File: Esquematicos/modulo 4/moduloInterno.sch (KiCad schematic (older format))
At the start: 15 parts

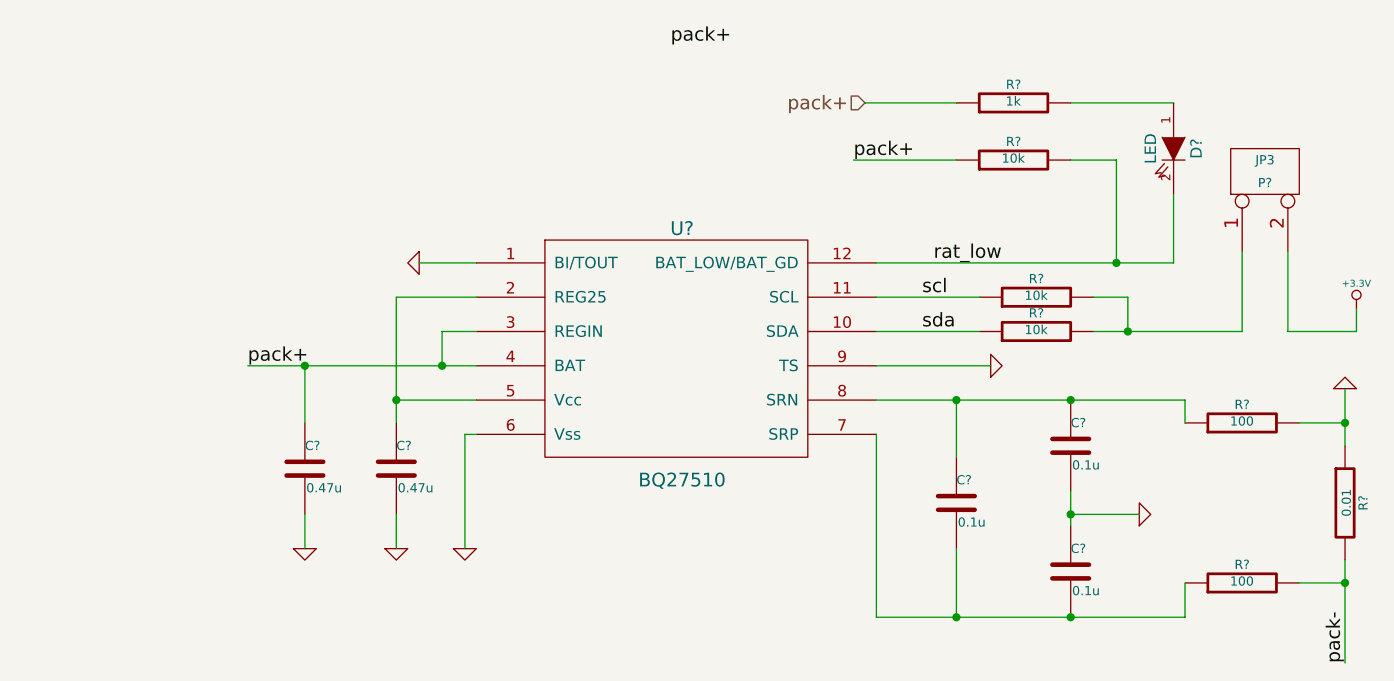
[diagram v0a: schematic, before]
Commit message: Esquematico terminado
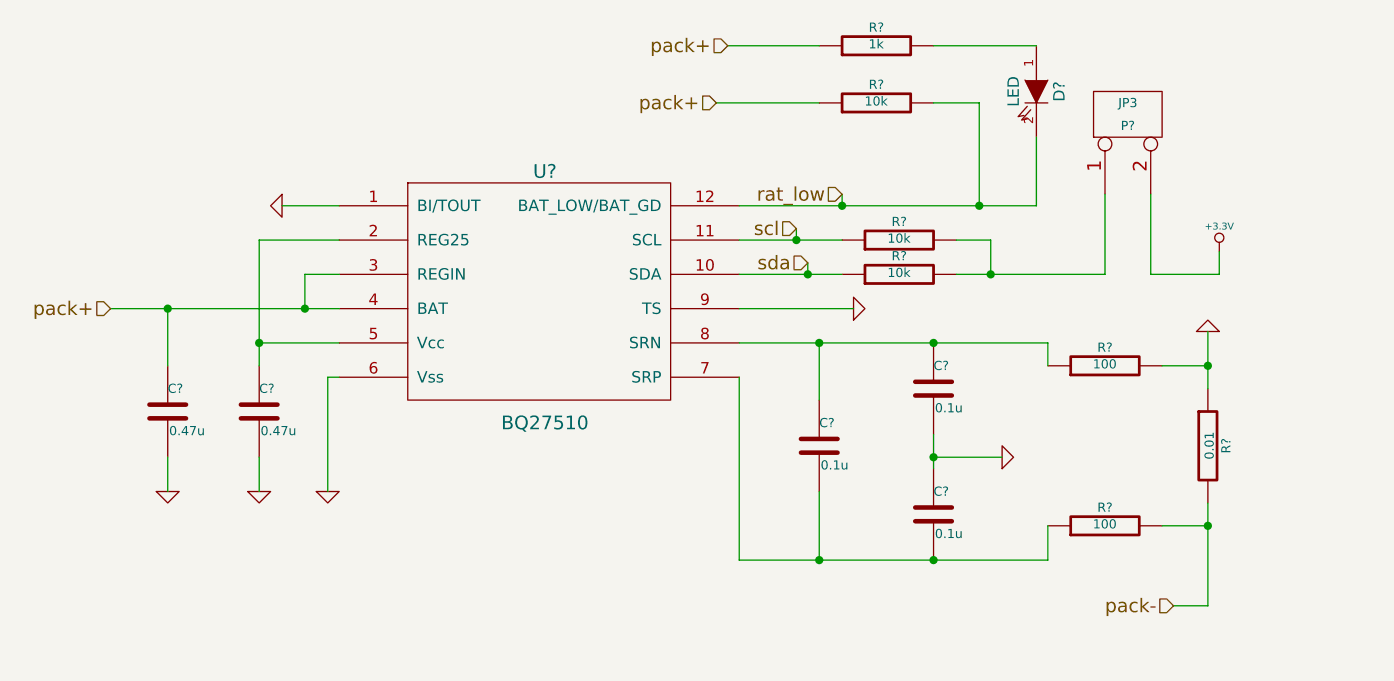
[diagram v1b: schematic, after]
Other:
- moved on the sheet: C?, D?, P?, R?, U?

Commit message: cambios
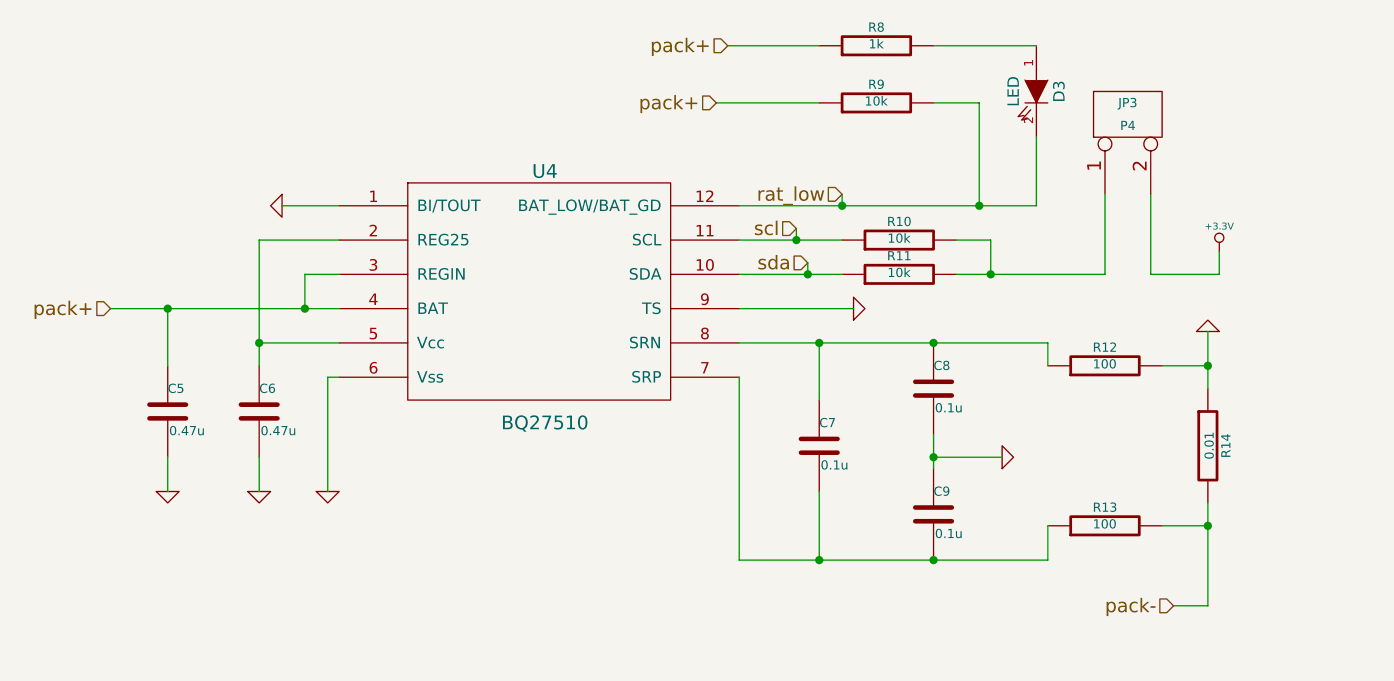
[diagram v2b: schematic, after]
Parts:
- gave numbers to parts that had none: 15
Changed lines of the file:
@@
 Sheet 2 3
 Title ""
-Date "18 feb 2014"
+Date "19 feb 2014"
 Rev ""
 Comp ""
@@
 $EndDescr
 $Comp
-L BQ27510 U?
+L BQ27510 U4
 U 1 1 52FE9FCC
 P 5050 3100
-F 0 "U?" H 5050 3500 60  0000 C CNN
+F 0 "U4" H 5050 3500 60  0000 C CNN
 F 1 "BQ27510" H 5050 2400 60  0000 C CNN
 F 2 "~" H 4850 3150 60  0000 C CNN
@@
 $EndComp
 $Comp
-L GND #PWR?
+L GND #PWR013
 U 1 1 52FE9FCD
 P 3900 2850
-F 0 "#PWR?" H 3900 2850 30  0001 C CNN
+F 0 "#PWR013" H 3900 2850 30  0001 C CNN
 F 1 "GND" H 3900 2780 30  0001 C CNN
 F 2 "" H 3900 2850 60  0000 C CNN
@@
 Connection ~ 4000 3300
 $Comp
-L C C?
+L C C5
 U 1 1 52FE9FCE
 P 3400 3750
-F 0 "C?" H 3400 3850 40  0000 L CNN
+F 0 "C5" H 3400 3850 40  0000 L CNN
 F 1 "0.47u" H 3406 3665 40  0000 L CNN
 F 2 "~" H 3438 3600 30  0000 C CNN
@@
 Connection ~ 3400 3300
 $Comp
-L C C?
+L C C6
 U 1 1 52FE9FCF
 P 3800 3750
-F 0 "C?" H 3800 3850 40  0000 L CNN
+F 0 "C6" H 3800 3850 40  0000 L CNN
 F 1 "0.47u" H 3806 3665 40  0000 L CNN
 F 2 "~" H 3838 3600 30  0000 C CNN
@@
 Connection ~ 3800 3450
 $Comp
-L GND #PWR?
+L GND #PWR014
 U 1 1 52FE9FD0
 P 3400 4100
-F 0 "#PWR?" H 3400 4100 30  0001 C CNN
+F 0 "#PWR014" H 3400 4100 30  0001 C CNN
 F 1 "GND" H 3400 4030 30  0001 C CNN
 F 2 "" H 3400 4100 60  0000 C CNN
@@
 $EndComp
 $Comp
-L GND #PWR?
+L GND #PWR015
 U 1 1 52FE9FD1
 P 3800 4100
-F 0 "#PWR?" H 3800 4100 30  0001 C CNN
+F 0 "#PWR015" H 3800 4100 30  0001 C CNN
 F 1 "GND" H 3800 4030 30  0001 C CNN
 F 2 "" H 3800 4100 60  0000 C CNN
@@
 $EndComp
 $Comp
-L GND #PWR?
+L GND #PWR016
 U 1 1 52FE9FD2
 P 4100 4100
-F 0 "#PWR?" H 4100 4100 30  0001 C CNN
+F 0 "#PWR016" H 4100 4100 30  0001 C CNN
 F 1 "GND" H 4100 4030 30  0001 C CNN
 F 2 "" H 4100 4100 60  0000 C CNN
@@
 	3400 3950 3400 4100
 $Comp
-L R R?
+L R R9
 U 1 1 52FE9FD3
 P 6500 2400
-F 0 "R?" V 6580 2400 40  0000 C CNN
+F 0 "R9" V 6580 2400 40  0000 C CNN
 F 1 "10k" V 6507 2401 40  0000 C CNN
 F 2 "~" V 6430 2400 30  0000 C CNN
@@
 $EndComp
 $Comp
-L R R?
+L R R8
 U 1 1 52FE9FD4
 P 6500 2150
-F 0 "R?" V 6580 2150 40  0000 C CNN
+F 0 "R8" V 6580 2150 40  0000 C CNN
 F 1 "1k" V 6507 2151 40  0000 C CNN
 F 2 "~" V 6430 2150 30  0000 C CNN
@@
 	5800 2400 6250 2400
 $Comp
-L LED D?
+L LED D3
 U 1 1 52FE9FD5
 P 7200 2350
-F 0 "D?" H 7200 2450 50  0000 C CNN
+F 0 "D3" H 7200 2450 50  0000 C CNN
 F 1 "LED" H 7200 2250 50  0000 C CNN
 F 2 "~" H 7200 2350 60  0000 C CNN
@@
 Connection ~ 6950 2850
 $Comp
-L R R?
+L R R10
 U 1 1 52FE9FD6
 P 6600 3000
-F 0 "R?" V 6680 3000 40  0000 C CNN
+F 0 "R10" V 6680 3000 40  0000 C CNN
 F 1 "10k" V 6607 3001 40  0000 C CNN
 F 2 "~" V 6530 3000 30  0000 C CNN
@@
 	5900 3000 6350 3000
 $Comp
-L R R?
+L R R11
 U 1 1 52FE9FD7
 P 6600 3150
-F 0 "R?" V 6680 3150 40  0000 C CNN
+F 0 "R11" V 6680 3150 40  0000 C CNN
 F 1 "10k" V 6607 3151 40  0000 C CNN
 F 2 "~" V 6530 3150 30  0000 C CNN
@@
 	7000 3000 7000 3150
 $Comp
-L CONN_2 P?
+L CONN_2 P4
 U 1 1 52FE9FD8
 P 7600 2450
-F 0 "P?" V 7550 2450 40  0000 C CNN
+F 0 "P4" V 7550 2450 40  0000 C CNN
 F 1 "JP3" V 7650 2450 40  0000 C CNN
 F 2 "" H 7600 2450 60  0000 C CNN
@@
 	7700 3150 8000 3150
 $Comp
-L +3.3V #PWR?
+L +3.3V #PWR017
 U 1 1 52FE9FD9
 P 8000 3050
-F 0 "#PWR?" H 8000 3010 30  0001 C CNN
+F 0 "#PWR017" H 8000 3010 30  0001 C CNN
 F 1 "+3.3V" H 8000 3160 30  0000 C CNN
 F 2 "" H 8000 3050 60  0000 C CNN
@@
 	8000 3150 8000 3050
 $Comp
-L GND #PWR?
+L GND #PWR018
 U 1 1 52FE9FDA
 P 6400 3300
-F 0 "#PWR?" H 6400 3300 30  0001 C CNN
+F 0 "#PWR018" H 6400 3300 30  0001 C CNN
 F 1 "GND" H 6400 3230 30  0001 C CNN
 F 2 "" H 6400 3300 60  0000 C CNN
@@
 	5900 3300 6400 3300
 $Comp
-L C C?
+L C C7
 U 1 1 52FE9FDB
 P 6250 3900
-F 0 "C?" H 6250 4000 40  0000 L CNN
+F 0 "C7" H 6250 4000 40  0000 L CNN
 F 1 "0.1u" H 6256 3815 40  0000 L CNN
 F 2 "~" H 6288 3750 30  0000 C CNN
@@
 	5900 3600 5900 4400
 $Comp
-L C C?
+L C C8
 U 1 1 52FE9FDC
 P 6750 3650
-F 0 "C?" H 6750 3750 40  0000 L CNN
+F 0 "C8" H 6750 3750 40  0000 L CNN
 F 1 "0.1u" H 6756 3565 40  0000 L CNN
 F 2 "~" H 6788 3500 30  0000 C CNN
@@
 Connection ~ 6250 3450
 $Comp
-L C C?
+L C C9
 U 1 1 52FE9FDD
 P 6750 4200
-F 0 "C?" H 6750 4300 40  0000 L CNN
+F 0 "C9" H 6750 4300 40  0000 L CNN
 F 1 "0.1u" H 6756 4115 40  0000 L CNN
 F 2 "~" H 6788 4050 30  0000 C CNN
@@
 	6750 3850 6750 4000
 $Comp
-L GND #PWR?
+L GND #PWR019
 U 1 1 52FE9FDE
 P 7050 3950
-F 0 "#PWR?" H 7050 3950 30  0001 C CNN
+F 0 "#PWR019" H 7050 3950 30  0001 C CNN
 F 1 "GND" H 7050 3880 30  0001 C CNN
 F 2 "" H 7050 3950 60  0000 C CNN
@@
 Connection ~ 6750 3950
 $Comp
-L R R?
+L R R12
 U 1 1 52FE9FDF
 P 7500 3550
-F 0 "R?" V 7580 3550 40  0000 C CNN
+F 0 "R12" V 7580 3550 40  0000 C CNN
 F 1 "100" V 7507 3551 40  0000 C CNN
 F 2 "~" V 7430 3550 30  0000 C CNN
@@
 $EndComp
 $Comp
-L R R?
+L R R13
 U 1 1 52FE9FE0
 P 7500 4250
-F 0 "R?" V 7580 4250 40  0000 C CNN
+F 0 "R13" V 7580 4250 40  0000 C CNN
 F 1 "100" V 7507 4251 40  0000 C CNN
 F 2 "~" V 7430 4250 30  0000 C CNN
@@
 Connection ~ 6750 3450
 $Comp
-L R R?
+L R R14
 U 1 1 52FE9FE1
 P 7950 3900
-F 0 "R?" V 8030 3900 40  0000 C CNN
+F 0 "R14" V 8030 3900 40  0000 C CNN
 F 1 "0.01" V 7957 3901 40  0000 C CNN
 F 2 "~" V 7880 3900 30  0000 C CNN
@@
 	7950 3400 7950 3650
 $Comp
-L GND #PWR?
+L GND #PWR020
 U 1 1 52FE9FE2
 P 7950 3400
-F 0 "#PWR?" H 7950 3400 30  0001 C CNN
+F 0 "#PWR020" H 7950 3400 30  0001 C CNN
 F 1 "GND" H 7950 3330 30  0001 C CNN
 F 2 "" H 7950 3400 60  0000 C CNN

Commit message: recuperacion
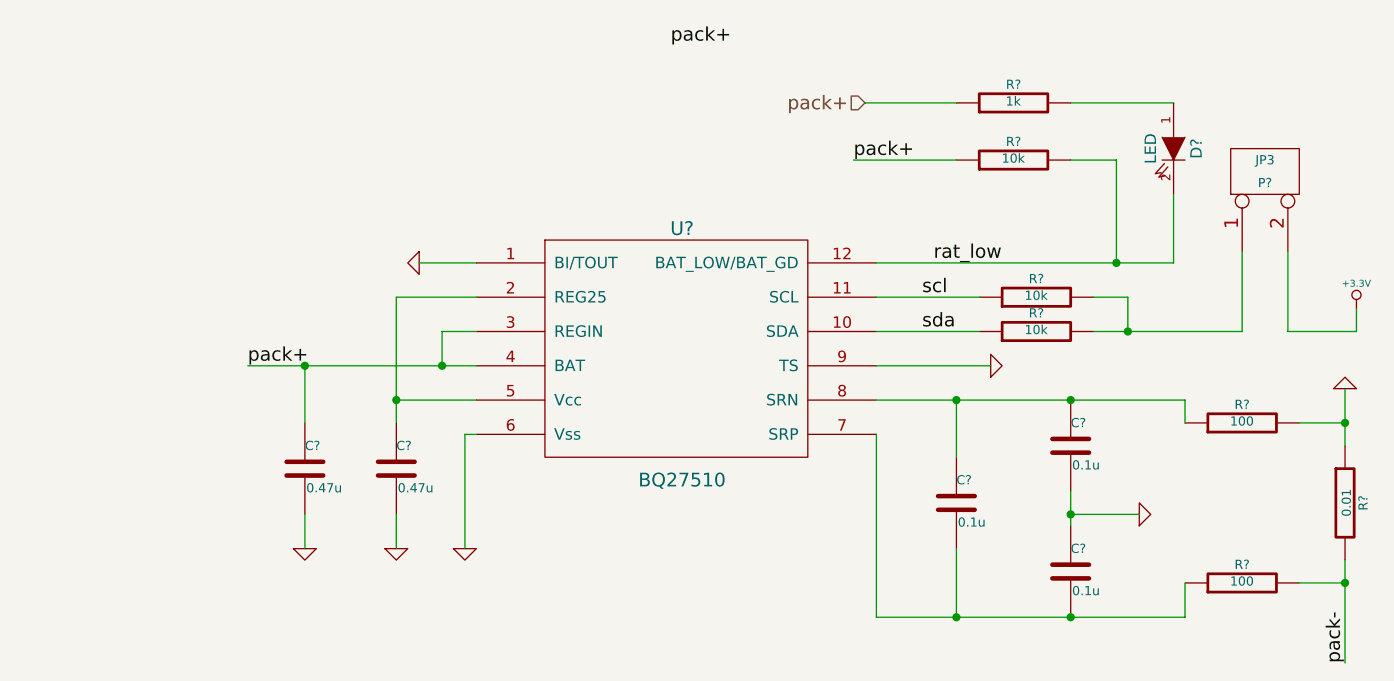
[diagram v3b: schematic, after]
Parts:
- renumbered C5 to C?, C6 to C?, C7 to C?, C8 to C?, C9 to C?, D3 to D?, P4 to P?, R9 to R?, R8 to R?, R10 to R?, R11 to R?, R12 to R?, R13 to R?, R14 to R?, U4 to U?
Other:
- moved on the sheet: C?, D?, P?, R?, U?
